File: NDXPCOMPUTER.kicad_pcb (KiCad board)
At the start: 2 copper layers, 34.6 x 58.9 mm, 6 parts, among them J2 USB_C_Receptacle_USB2.0_16P, U1 STM32H723VGTx, U2 BMI088, U3 LSM6DSM, U4 BMP280, U5 NEO-M9N

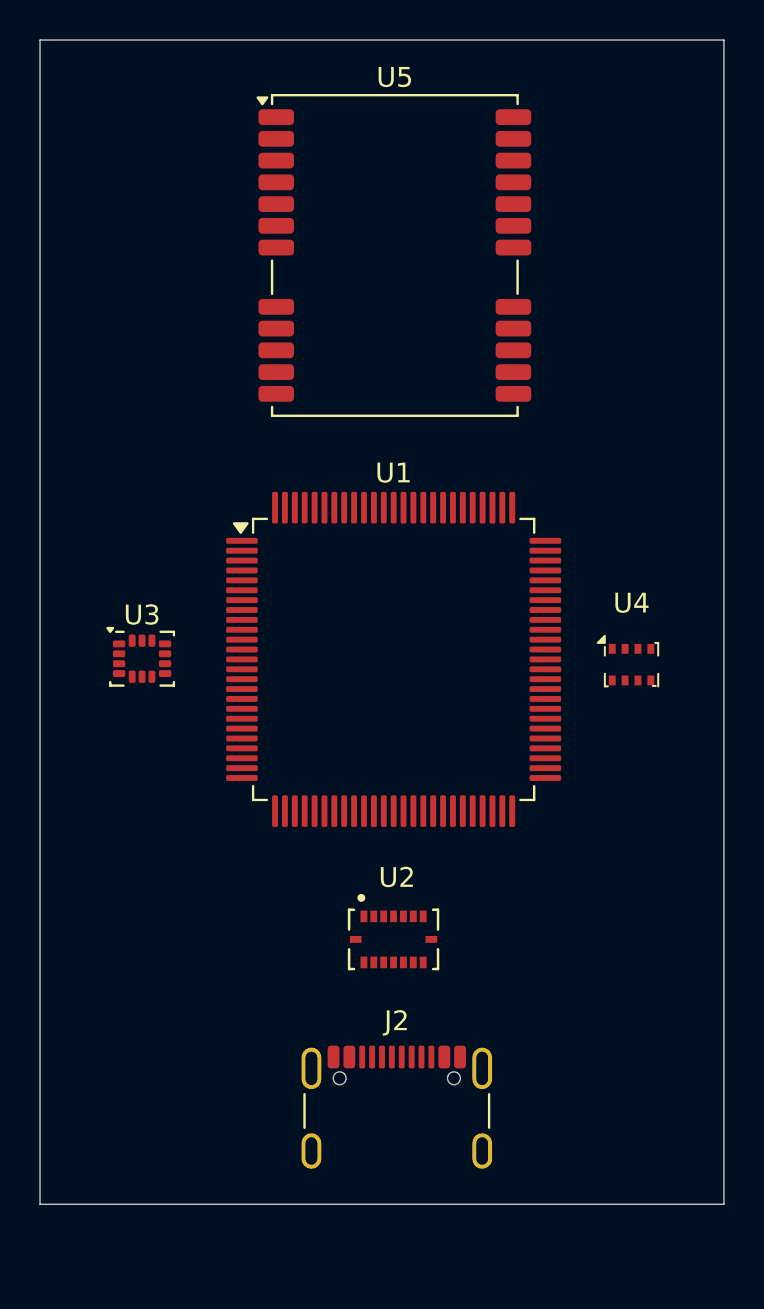
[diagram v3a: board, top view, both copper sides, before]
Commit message: Magnetometer🧲
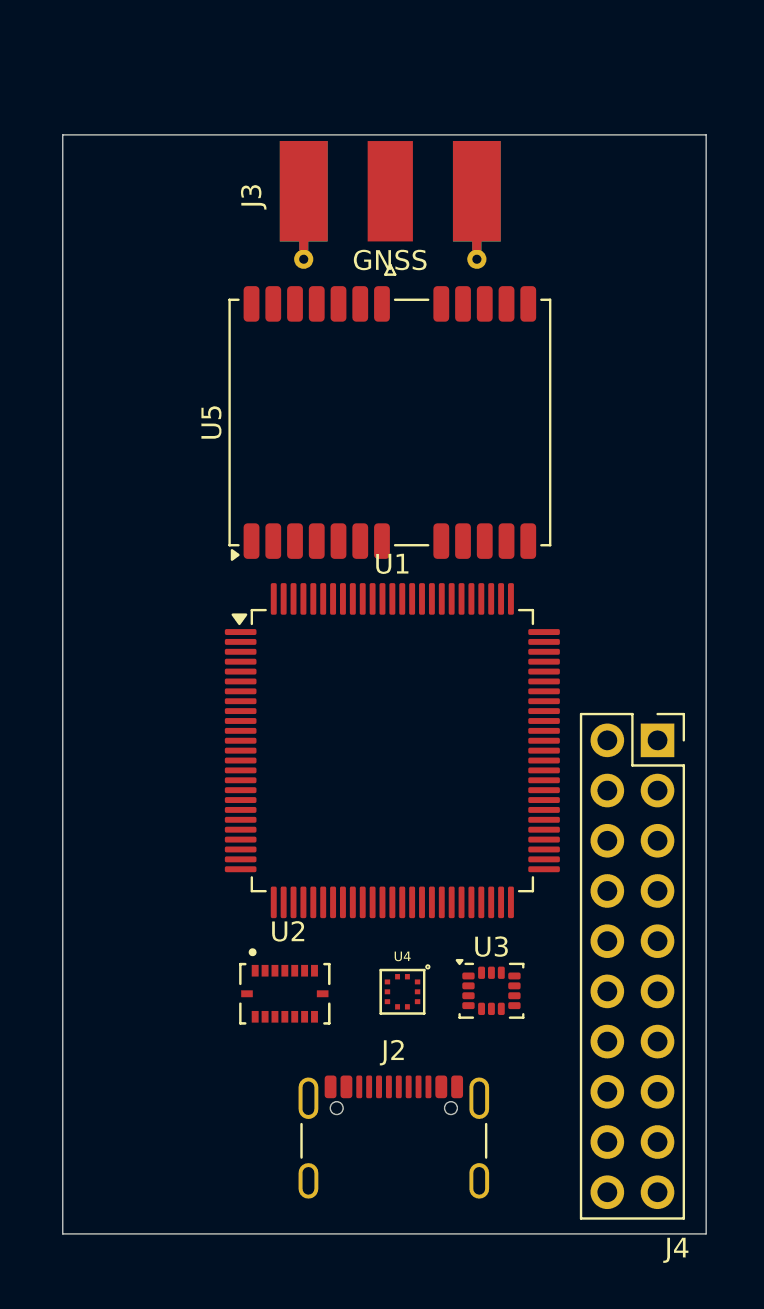
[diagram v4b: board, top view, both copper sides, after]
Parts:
- added G***: LOGO, Images:ND, F.Cu at (151.5, 75.2)
- added J3: Conn_Coaxial, Connector_Coaxial:SMA_Molex_73251-1153_EdgeMount_Horizontal, F.Cu at (139.9, 75.8)
- added J4: Conn_02x10_Counter_Clockwise, Connector_PinSocket_2.54mm:PinSocket_2x10_P2.54mm_Vertical, F.Cu at (153.4, 101.9)
- U4: value BMP280 -> BMP581; footprint Package_LGA:Bosch_LGA-8_2x2.5mm_P0.65mm_ClockwisePinNumbering -> BMP581:BMP581
- moved U3 24.4 mm to (145.0, 114.5)
- moved U4 20.2 mm to (140.5, 114.6)
- moved U5 8.45 mm to (139.9, 85.8), turned to 90 degrees
- moved U2 6.15 mm to (134.6, 114.7)
- moved U1 4.62 mm to (140.0, 102.4)
- moved J2 1.52 mm to (140.1, 123.1)
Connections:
- J2 pad A6: unconnected-(J2-D+-PadA6) -> D+
- J2 pad A7: unconnected-(J2-D--PadA7) -> D-
- J2 pad B5: unconnected-(J2-CC2-PadB5) -> Net-(J2-CC2)
- J2 pad B6: unconnected-(J2-D+-PadB6) -> D+
- J2 pad B7: unconnected-(J2-D--PadB7) -> D-
- U1 pad 10: Net-(U1-VSS-Pad10) -> GND
- U1 pad 100: unconnected-(U1-VDD-Pad100) -> +3.3V
- U1 pad 11: unconnected-(U1-VDD-Pad11) -> +3.3V
- U1 pad 12: unconnected-(U1-PH0-Pad12) -> GND
- U1 pad 14: unconnected-(U1-NRST-Pad14) -> Net-(U1-NRST)
- U1 pad 19: unconnected-(U1-VSSA-Pad19) -> GND
- U1 pad 20: unconnected-(U1-VREF+-Pad20) -> +3.3V
- U1 pad 21: unconnected-(U1-VDDA-Pad21) -> +3.3V
- U1 pad 26: Net-(U1-VSS-Pad10) -> GND
- U1 pad 27: unconnected-(U1-VDD-Pad27) -> +3.3V
- U1 pad 41: unconnected-(U1-PE11-Pad41) -> /NEO-M9N/CS_GPS
- U1 pad 42: unconnected-(U1-PE12-Pad42) -> /NEO-M9N/CLK_GPS
- U1 pad 43: unconnected-(U1-PE13-Pad43) -> /NEO-M9N/DO_GPS
- U1 pad 44: unconnected-(U1-PE14-Pad44) -> /NEO-M9N/DI_GPS
- U1 pad 48: unconnected-(U1-VCAP-Pad48) -> Net-(C11-Pad2)
- U1 pad 49: Net-(U1-VSS-Pad10) -> GND
- U1 pad 50: unconnected-(U1-VDD-Pad50) -> +3.3V
- U1 pad 6: unconnected-(U1-VBAT-Pad6) -> +3.3V
- U1 pad 69: unconnected-(U1-PA10-Pad69) -> Net-(U1-PA10)
- U1 pad 70: unconnected-(U1-PA11-Pad70) -> Net-(U1-PA11)
- U1 pad 73: unconnected-(U1-VCAP-Pad73) -> Net-(C12-Pad2)
- U1 pad 74: Net-(U1-VSS-Pad10) -> GND
- U1 pad 75: unconnected-(U1-VDD-Pad75) -> +3.3V
- U1 pad 94: unconnected-(U1-BOOT0-Pad94) -> Net-(U1-BOOT0)
- U1 pad 99: Net-(U1-VSS-Pad10) -> GND
- U3 pad 1: unconnected-(U3-SDO/SA0-Pad1) -> /LSM6DSM/SDO_IMU_LOW
- U3 pad 12: unconnected-(U3-CS-Pad12) -> /LSM6DSM/CS_IMU_LOW
- U3 pad 13: unconnected-(U3-SCL-Pad13) -> /LSM6DSM/SCL_IMU_LOW
- U3 pad 14: unconnected-(U3-SDA-Pad14) -> /LSM6DSM/SDI_IMU_LOW
- U3 pad 2: unconnected-(U3-SDX-Pad2) -> GND
- U3 pad 3: unconnected-(U3-SCX-Pad3) -> GND
- U3 pad 4: unconnected-(U3-INT1-Pad4) -> /LSM6DSM/INT_IMU_LOW
- U3 pad 5: unconnected-(U3-VDDIO-Pad5) -> +3.3V
- U3 pad 6: Net-(U3-GND-Pad6) -> GND
- U3 pad 7: Net-(U3-GND-Pad6) -> GND
- U3 pad 8: unconnected-(U3-VDD-Pad8) -> +3.3V
- U4 pad 1: unconnected-(U4-GND-Pad1) -> +3.3V
- U4 pad 2: unconnected-(U4-CSB-Pad2) -> /BMP581/SCK_BARO
- U4 pad 3: unconnected-(U4-SDI-Pad3) -> GND
- U4 pad 4: unconnected-(U4-SCK-Pad4) -> /BMP581/SDI_BARO
- U4 pad 5: unconnected-(U4-SDO-Pad5) -> /BMP581/SDO_BARO
- U4 pad 6: unconnected-(U4-VDDIO-Pad6) -> /BMP581/CS_BARO
- U4 pad 7: unconnected-(U4-GND-Pad7) -> /BMP581/INT_BARO
- U4 pad 8: unconnected-(U4-VDD-Pad8) -> GND
- U5 pad 1: unconnected-(U5-~{SAFEBOOT}-Pad1) -> Net-(U5-~{SAFEBOOT})
- U5 pad 10: Net-(U5-GND-Pad10) -> GND
- U5 pad 11: unconnected-(U5-RF_IN-Pad11) -> Net-(J3-In)
- U5 pad 12: Net-(U5-GND-Pad10) -> GND
- U5 pad 13: Net-(U5-GND-Pad10) -> GND
- U5 pad 18: unconnected-(U5-SDA/~{SPI_CS}-Pad18) -> /NEO-M9N/CS_GPS
- U5 pad 19: unconnected-(U5-SCL/SPI_CLK-Pad19) -> /NEO-M9N/CLK_GPS
- U5 pad 2: unconnected-(U5-D_SEL-Pad2) -> GND
- U5 pad 20: unconnected-(U5-TXD/SPI_MISO-Pad20) -> /NEO-M9N/DO_GPS
- U5 pad 21: unconnected-(U5-RXD/SPI_MOSI-Pad21) -> /NEO-M9N/DI_GPS
- U5 pad 22: unconnected-(U5-V_BCKP-Pad22) -> +3.3V
- U5 pad 23: unconnected-(U5-VCC-Pad23) -> +3.3V
- U5 pad 24: Net-(U5-GND-Pad10) -> GND
- U5 pad 7: unconnected-(U5-VDD_USB-Pad7) -> GND
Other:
- board size 34.6 x 58.9 mm -> 32.6 x 55.6 mm
- board text added: "GNSS"
